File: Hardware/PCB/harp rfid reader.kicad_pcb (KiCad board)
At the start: 4 copper layers, 45 x 26.5 mm, 51 parts, among them IC1 FT232RL, IC2 LP5907MFX-3.3, IC3 ATxmega32A4U-A, IC4 741G126DBVAHC, J1 USB4105-GF-A, J2 OUT0, Q1 BC817-40W, Q2 NTF2955T1G, U1 ID-12/20SMD

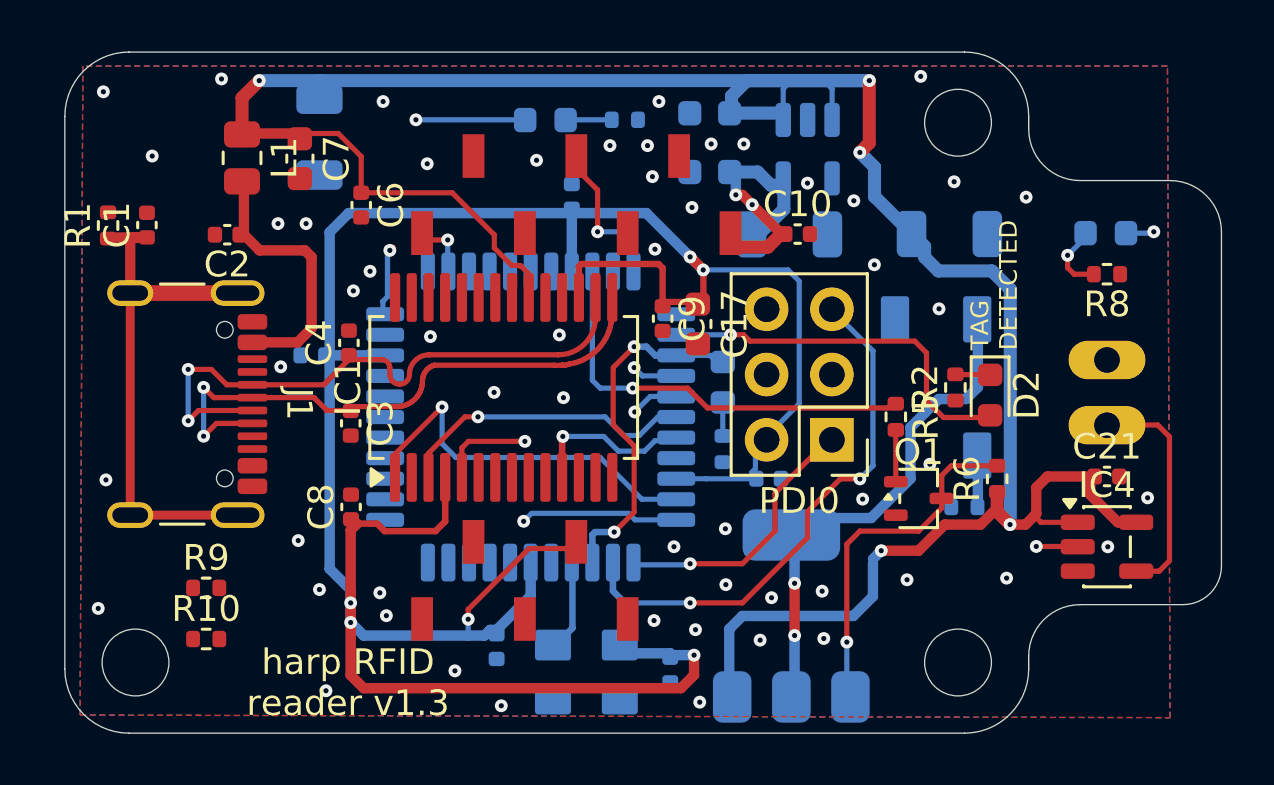
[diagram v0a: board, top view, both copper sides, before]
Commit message: versão 1.3 final & ficheiros de manufacturing
- ainda sem revisão do Filipe
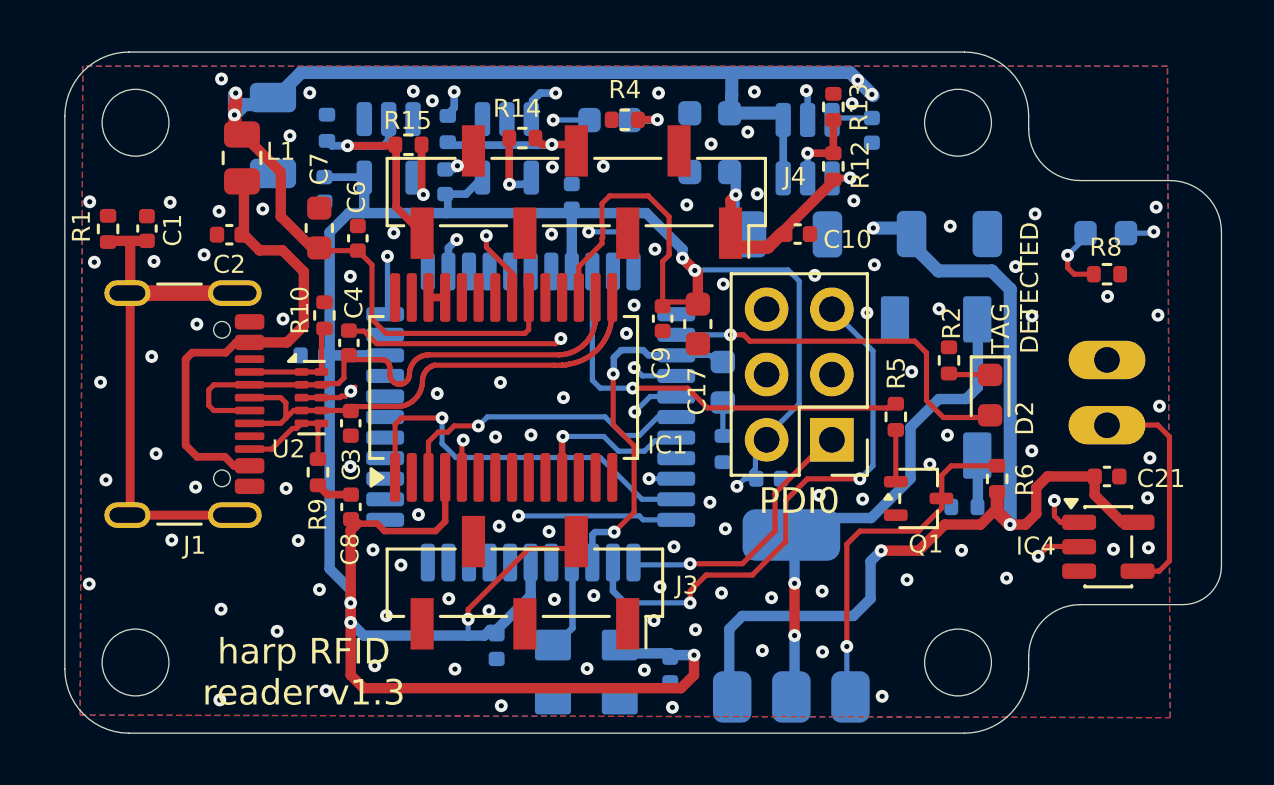
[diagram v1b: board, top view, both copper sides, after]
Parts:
- added C22: 100nF, Capacitor_SMD:C_0402_1005Metric, B.Cu at (136.1, 97.1)
- added C23: 10n, Capacitor_SMD:C_0402_1005Metric, B.Cu at (157.4, 94.8)
- added C30: 100nF, Capacitor_SMD:C_0402_1005Metric, B.Cu at (140.8, 96.8)
- added IC10: SN74LVC1G125DBVT, Package_TO_SOT_SMD:SOT-23-5, B.Cu at (143.2, 95.5)
- added IC5: SN74LVC1G125DBVT, Package_TO_SOT_SMD:SOT-23-5, B.Cu at (138.6, 95.5)
- added J3: NPPN051BFLD-RC, Connector_PinSocket_2.00mm:PinSocket_1x05_P2.00mm_Vertical_SMD_Pin1Right, F.Cu at (143.9, 112.4)
- added J4: NPPN071BFLC-RC, Connector_PinSocket_2.00mm:PinSocket_1x07_P2.00mm_Vertical_SMD_Pin1Right, F.Cu at (145.9, 97.2)
- added R11: 10k, Resistor_SMD:R_0402_1005Metric, B.Cu at (136.2, 94.7)
- added R12: 22k, Resistor_SMD:R_0402_1005Metric, F.Cu at (155.9, 96.2)
- added R13: 10k, Resistor_SMD:R_0402_1005Metric, F.Cu at (155.9, 93.9)
- added R14: 0R, Resistor_SMD:R_0402_1005Metric, F.Cu at (143.8, 95.1)
- added R15: 0R, Resistor_SMD:R_0402_1005Metric, F.Cu at (139.4, 95.4)
- added R16: 10k, Resistor_SMD:R_0402_1005Metric, B.Cu at (140.9, 94.8)
- added U2: TPD4E05U06DQA, Package_SON:USON-10_2.5x1.0mm_P0.5mm, F.Cu at (135.6, 105.2)
- added UNK_HOLE_2: , dummyfp2, F.Cu at (128.8, 94.5)
- D1: value TAG_B0 -> 5975004407F
- D2: value TAG_T0 -> 5975004407F
- D3: value STATE -> 5975004407F
- D4: value OUTLED -> 5975004407F
- IC2: value LP5907MFX-3.3 -> NJM11100F1-TE2; footprint Package_TO_SOT_SMD:TSOT-23-5 -> Package_TO_SOT_SMD:SOT-23-6
- IC4: value 741G126DBVAHC -> SN74LVC1G125DBVT
- J2: value OUT0 -> 282834-2
- L1: value 40R@100MHz -> MI0805K400R-10
- PDI0: value MA03-2 -> 67996-206HLF
- R4: moved to F.Cu
- R7: value 75 >1/4W -> 39R
- SP1: value BUZZER-COIL_SMT-0540-S-R -> SMT-0540-S-R
- U1: footprint harp rfid reader:ID-12_SMD -> harp rfid reader:ID-12_SMD body
- X1: renamed from OSC1; value CNP-MISCELLANEOUS_OSCILLATOR -> O 32,0-JT32C-A-K-3,3-LF
- moved U1 18.7 mm to (145.3, 104.8), turned to 180 degrees
- moved R10 13.4 mm to (136.1, 102.0), turned to 90 degrees
- moved R9 6.26 mm to (135.8, 108.1), turned to -90 degrees
- moved C7 2.80 mm to (135.9, 98.6), turned to 90 degrees
- moved D1 2.50 mm to (147.2, 94.4)
- moved C20 1.81 mm to (134.1, 95.0)
- moved C6 1.30 mm to (137.4, 99.0), turned to 90 degrees
- moved R2 1.08 mm to (160.4, 103.8), turned to -90 degrees
- moved C1 0.13 mm to (129.2, 98.6)
- moved R1 0.13 mm to (127.7, 98.6)
- moved J1 0.11 mm to (129.5, 105.5)
- moved C2 0.08 mm to (132.4, 98.9)
- moved IC4 0.05 mm to (166.6, 111.0)
- turned R4 to 0 degrees
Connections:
- net Net-(J1-CC1) renamed /CC2
- net Net-(J1-CC2) renamed /CC1
- C10 pad 1: +3V3 -> VRFID
- C11 pad 1: +3V3 -> VRFID
- C12 pad 1: VDDIO -> +3V3
- C13 pad 1: VDDIO -> +3V3
- C14 pad 1: VDDIO -> +3V3
- C15 pad 1: VDDIO -> +3V3
- C16 pad 1: VDDIO -> +3V3
- C17 pad 1: VDDIO -> +3V3
- C18 pad 1: +3V3 -> VRFID
- C8 pad 1: VDDIO -> +3V3
- C9 pad 1: VDDIO -> +3V3
- IC1 pad 17: VDDIO -> +3V3
- IC1 pad 4: VDDIO -> +3V3
- IC2 pad 3: +5V -> Net-(IC2-NoiseBypass)
- IC2 pad 4: unconnected-(IC2-N/C-Pad4) -> VRFID
- IC2 pad 5: +3V3 -> Net-(IC2-Vadj)
- IC3 pad 13: /core/F2 -> /core/UC_F2
- IC3 pad 19: VDDIO -> +3V3
- IC3 pad 22: /core/TX -> /core/UC_TX
- IC3 pad 31: VDDIO -> +3V3
- IC3 pad 39: VDDIO -> +3V3
- IC3 pad 9: VDDIO -> +3V3
- IC4 pad 1: +5V -> GND
- PDI0 pad 2: VDDIO -> +3V3
- X1 pad 4: VDDIO -> +3V3
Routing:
- net +3V3: track 10.8 -> 117.9 mm, vias 2 -> 8
- net VDDIO: track 104.9 -> 0.00 mm, vias 6 -> 0
- net GND: track 0.00 -> 21.8 mm, vias 53 -> 109
- net VRFID: track 0.00 -> 11.7 mm, vias 0 -> 2
- net /core/UC_TX: track 0.00 -> 10.5 mm, vias 0 -> 2
- net V USB: track 10.4 -> 18.3 mm
- net /core/F2: track 2.24 -> 9.53 mm
- net /core/UC_F2: track 0.00 -> 7.06 mm, vias 0 -> 2
- net /CC1: track 0.00 -> 4.66 mm
- net /core/DETECT1: track 12.4 -> 17.1 mm, vias 2 -> 3
- net /CC2: track 0.00 -> 4.53 mm
- net /USBD+: track 23.2 -> 19.1 mm, vias 2 -> 0
- net Net-(IC2-Vadj): track 0.00 -> 3.20 mm, vias 0 -> 1
- net +5V: track 102.8 -> 99.6 mm, vias 5 -> 7
- net /USBD-: track 24.1 -> 21.3 mm, vias 2 -> 0
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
